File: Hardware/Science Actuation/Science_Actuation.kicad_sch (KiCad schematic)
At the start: 79 parts, among them J2 RJ45_LED_Shielded, SW1 SW_Push, SW10 SW_SPDT, SW2 SW_Push, SW3 SW_Push, SW4 SW_Push, SW5 SW_Push, SW6 SW_Push, SW7 SW_Push, U2 OKI, U2 Teensy4.1_DEV-16771

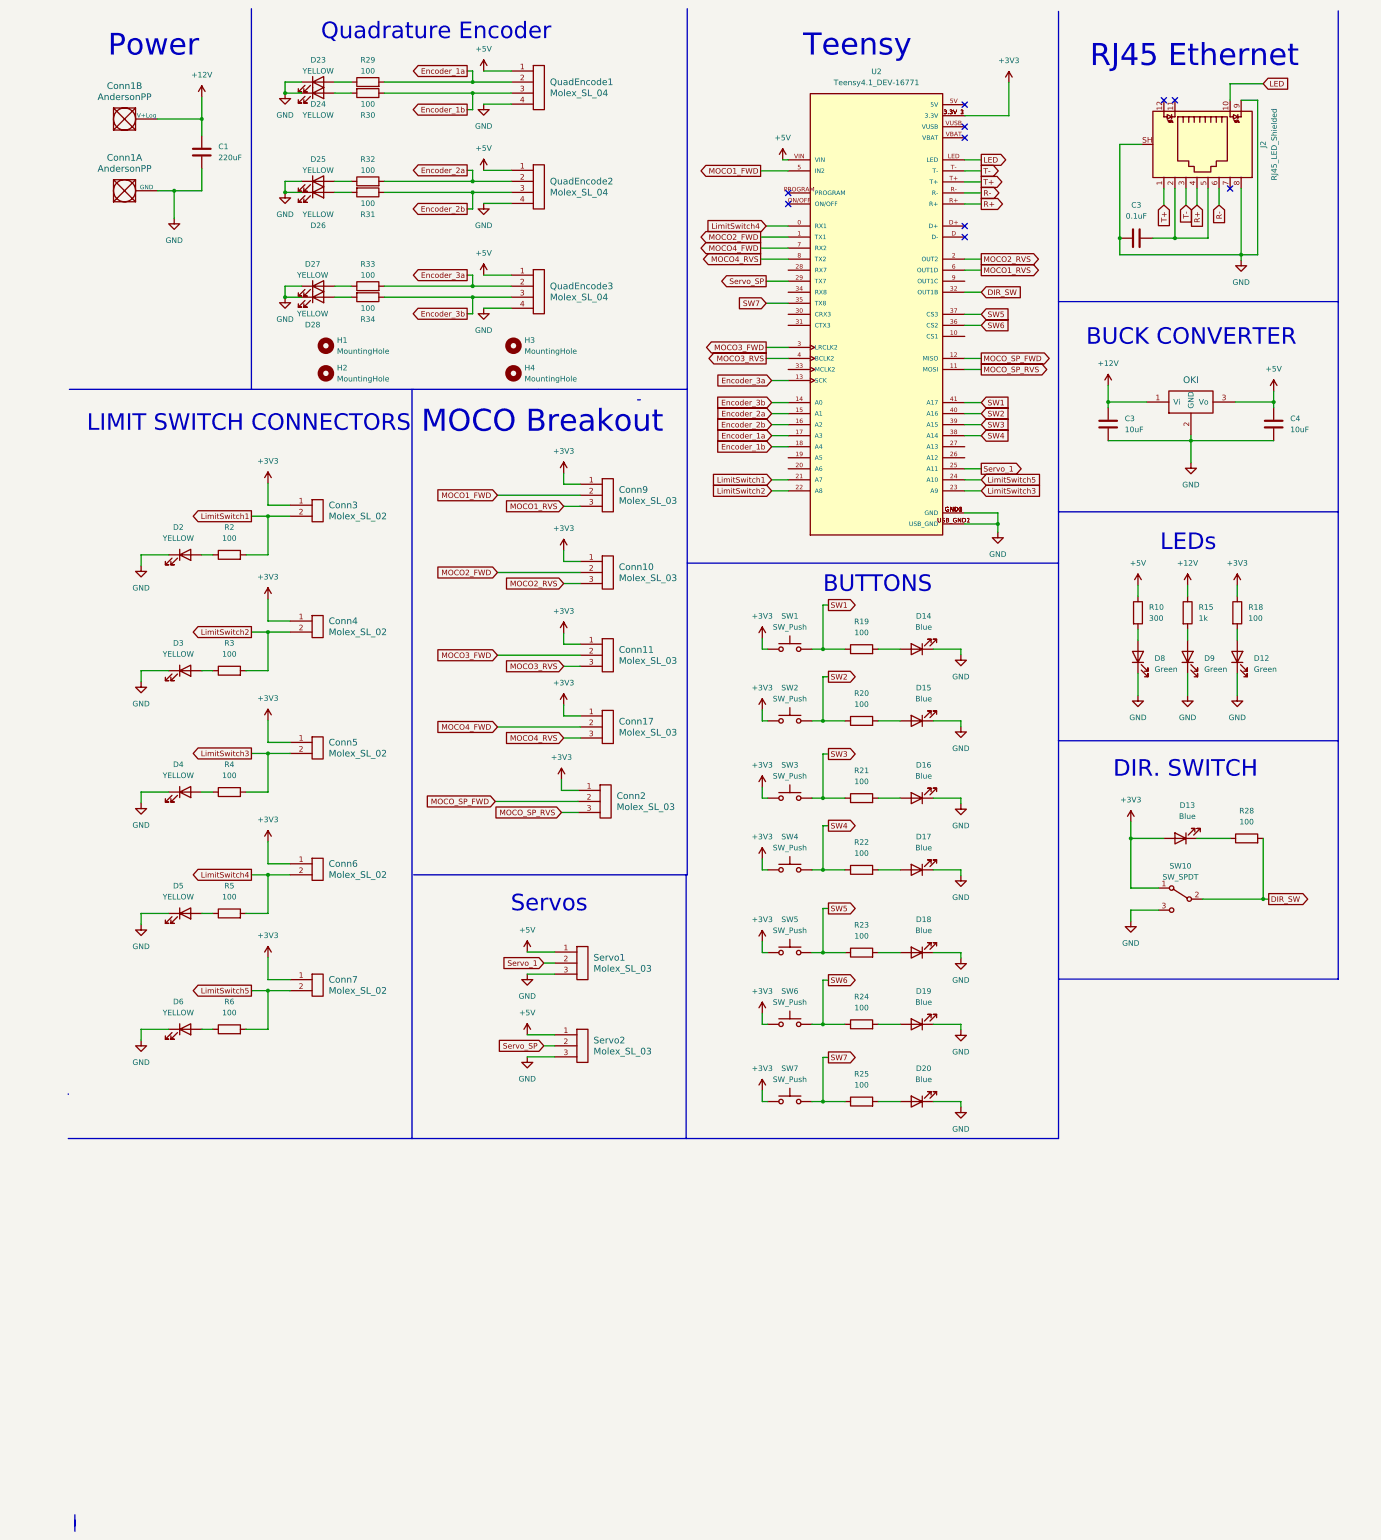
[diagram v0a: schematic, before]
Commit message: Updated Science Actuation again (definitely not finished)
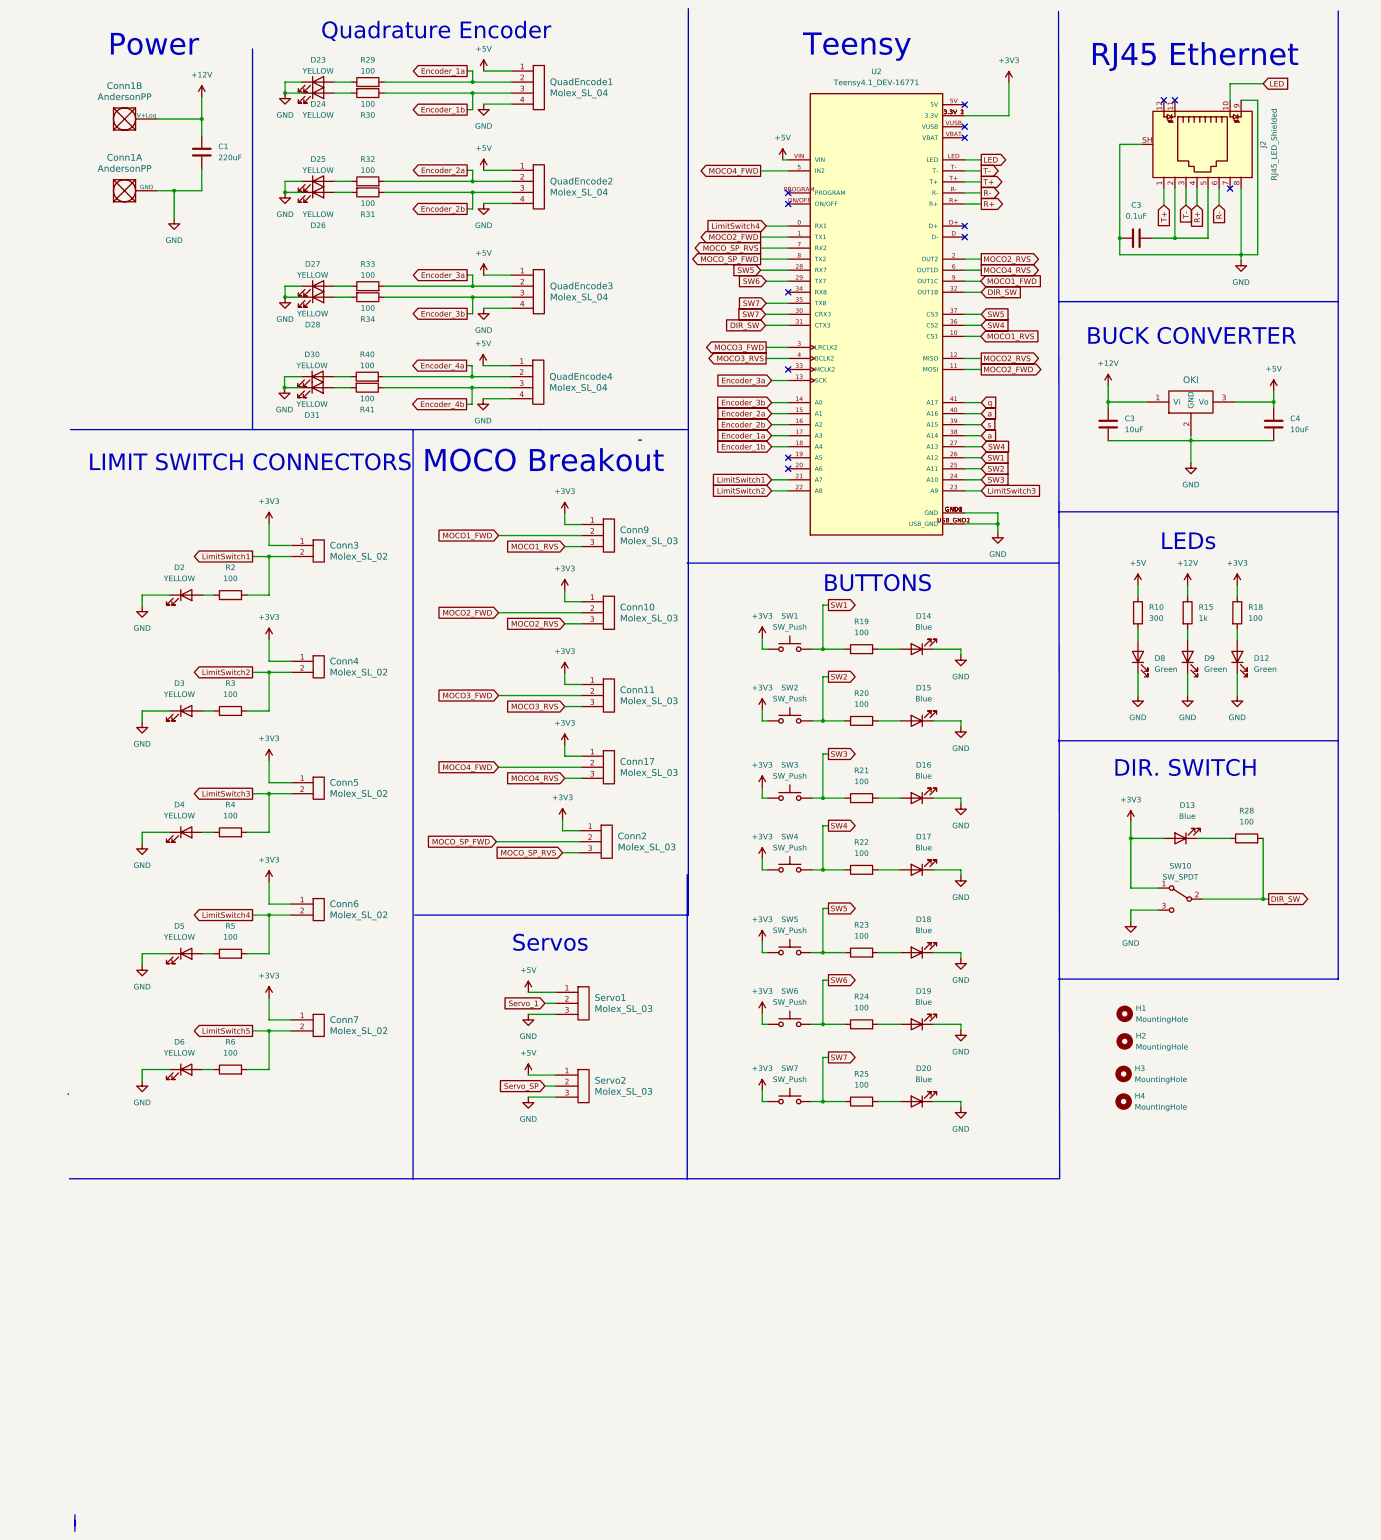
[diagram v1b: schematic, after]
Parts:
- added D30, D31: YELLOW, LED_SMD:LED_0603_1608Metric_Pad1.05x0.95mm_HandSolder, symbol Device:LED
- added QuadEncode4: Molex_SL_04, MRDT_Connectors:MOLEX_SL_04_Vertical, symbol MRDT_Connectors:Molex_SL_04
- added R40, R41: 100, Resistor_SMD:R_0603_1608Metric_Pad0.98x0.95mm_HandSolder, symbol Device:R
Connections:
- net +5V: now also QuadEncode4.1
- net DIR_SW: now also U2.31 (CTX3)
- net GND: now also D30.1 (K), D31.1 (K), QuadEncode4.4
- net LimitSwitch5: no longer U2.24 (A10)
- net MOCO1_FWD: now also U2.9 (OUT1C); no longer U2.5 (IN2)
- net MOCO1_RVS: now also U2.10 (CS1); no longer U2.6 (OUT1D)
- net MOCO2_FWD: now also U2.11 (MOSI)
- net MOCO2_RVS: now also U2.12 (MISO)
- net MOCO4_FWD: now also U2.5 (IN2); no longer U2.7 (RX2)
- net MOCO4_RVS: now also U2.6 (OUT1D); no longer U2.8 (TX2)
- net MOCO_SP_FWD: now also U2.8 (TX2); no longer U2.12 (MISO)
- net MOCO_SP_RVS: now also U2.7 (RX2); no longer U2.11 (MOSI)
- net SW1: now also U2.26 (A12); no longer U2.41 (A17)
- net SW2: now also U2.25 (A11); no longer U2.40 (A16)
- net SW3: now also U2.24 (A10); no longer U2.39 (A15)
- net SW4: now also U2.27 (A13), U2.36 (CS2); no longer U2.38 (A14)
- net SW5: now also U2.28 (RX7)
- net SW6: now also U2.29 (TX7); no longer U2.36 (CS2)
- net SW7: now also U2.30 (CRX3)
- net Servo_1: no longer U2.25 (A11)
- net Servo_SP: no longer U2.29 (TX7)
- new net: D30.2 (A), R40.1
- new net: D31.2 (A), R41.2
- new net Encoder_4a: QuadEncode4.2, R40.2
- new net Encoder_4b: QuadEncode4.3, R41.1
- new net a: U2.38 (A14), U2.40 (A16)
- new net q: U2.41 (A17)
- new net s: U2.39 (A15)
- no-connect marks 10 -> 14
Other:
- moved on the sheet: Conn10, Conn11, Conn17, Conn2, Conn3, Conn4, Conn5, Conn6, Conn7, Conn9, D2, D3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
